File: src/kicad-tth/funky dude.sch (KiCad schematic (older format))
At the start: 30 parts, among them P1 CONN_2, P2 CONN_2, P3 CONN_2, U1 TLC2262

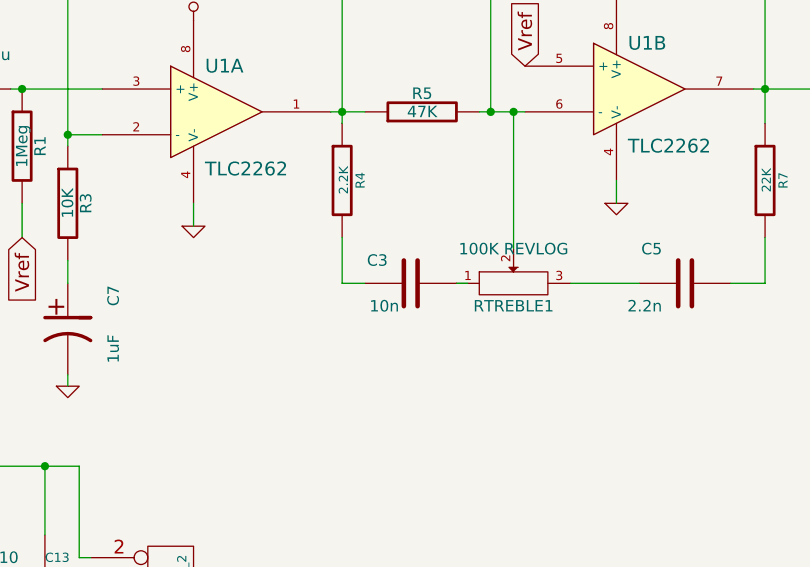
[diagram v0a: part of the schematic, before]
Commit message: pcb changes
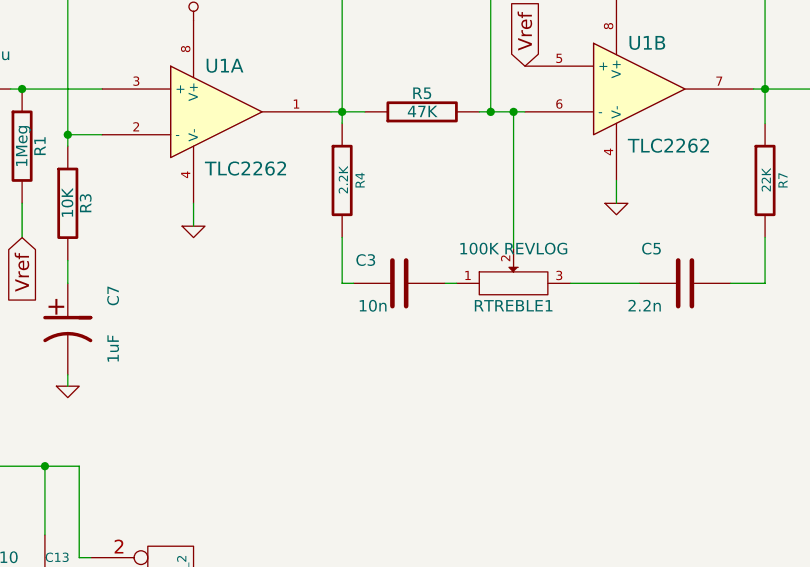
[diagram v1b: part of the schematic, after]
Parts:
- C13: footprint (none) -> Custom:C2-LARGE_PADS
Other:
- moved on the sheet: C3
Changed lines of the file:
@@
 Wire Wire Line
 	7800 3500 7800 3400
-Wire Wire Line
-	7650 5750 7700 5750
 Connection ~ 9000 4100
 Connection ~ 9000 4900
 Wire Wire Line
 	9000 3950 9000 5050
-Wire Wire Line
-	7150 5750 7250 5750
 Connection ~ 7800 4100
 Wire Wire Line
@@
 L C C3
 U 1 1 5194A4FE
-P 7450 5750
-F 0 "C3" V 7550 5850 50  0000 L CNN
-F 1 "10n" V 7350 5800 50  0000 L CNN
-F 2 "Custom:C2-LARGE_PADS" H 7450 5750 60  0001 C CNN
-F 3 "" H 7450 5750 60  0001 C CNN
-	1    7450 5750
+P 7400 5750
+F 0 "C3" V 7500 5850 50  0000 L CNN
+F 1 "10n" V 7300 5800 50  0000 L CNN
+F 2 "Custom:C2-LARGE_PADS" H 7400 5750 60  0001 C CNN
+F 3 "" H 7400 5750 60  0001 C CNN
+	1    7400 5750
 	0    -1   -1   0
 $EndComp
@@
 F 0 "C13" H 5850 7150 40  0000 L CNN
 F 1 "100n" H 5856 6965 40  0000 L CNN
-F 2 "" H 5888 6900 30  0000 C CNN
+F 2 "Custom:C2-LARGE_PADS" H 5888 6900 30  0001 C CNN
 F 3 "~" H 5850 7050 60  0000 C CNN
 	1    5850 7050
@@
 	9200 4500 9400 4500
 Connection ~ 9400 4500
+Wire Wire Line
+	7150 5750 7200 5750
+Wire Wire Line
+	7650 5750 7600 5750
 $EndSCHEMATC
